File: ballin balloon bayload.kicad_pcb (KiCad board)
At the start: 4 copper layers, 73 x 86 mm, 13 parts, among them J1 Molex 0510211000, J2 Molex 0532611071, J3 Molex 0510211000, J4 Conn_01x06_Pin, J5 Conn_01x06_Pin, U1 MICROSD_SPI_OR_SDIO_CARD, U2 3073, U3 2472

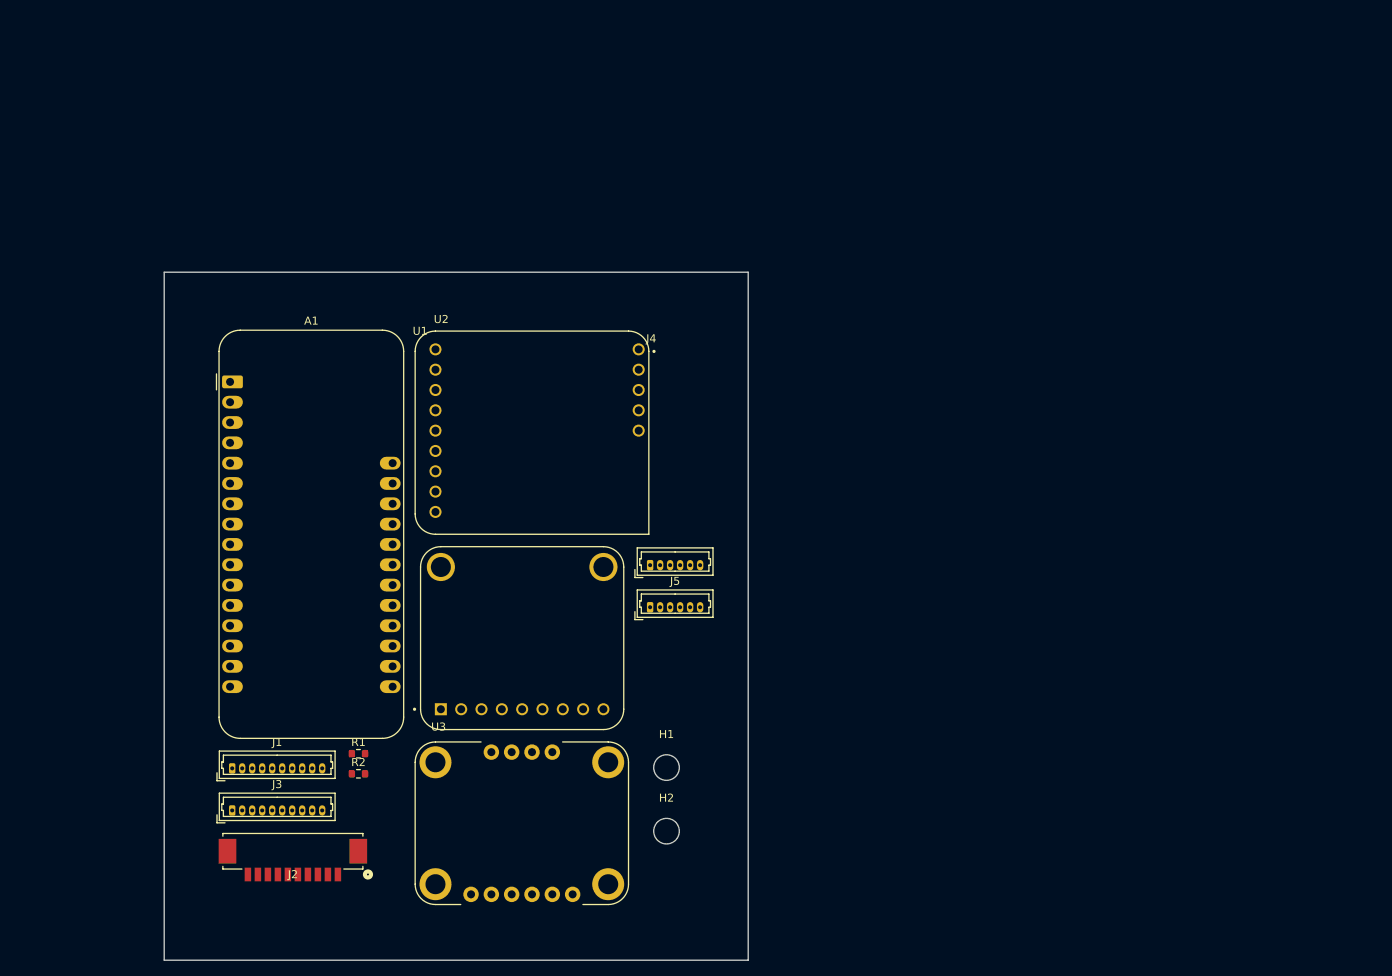
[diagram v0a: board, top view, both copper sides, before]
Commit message: updated pcb layout
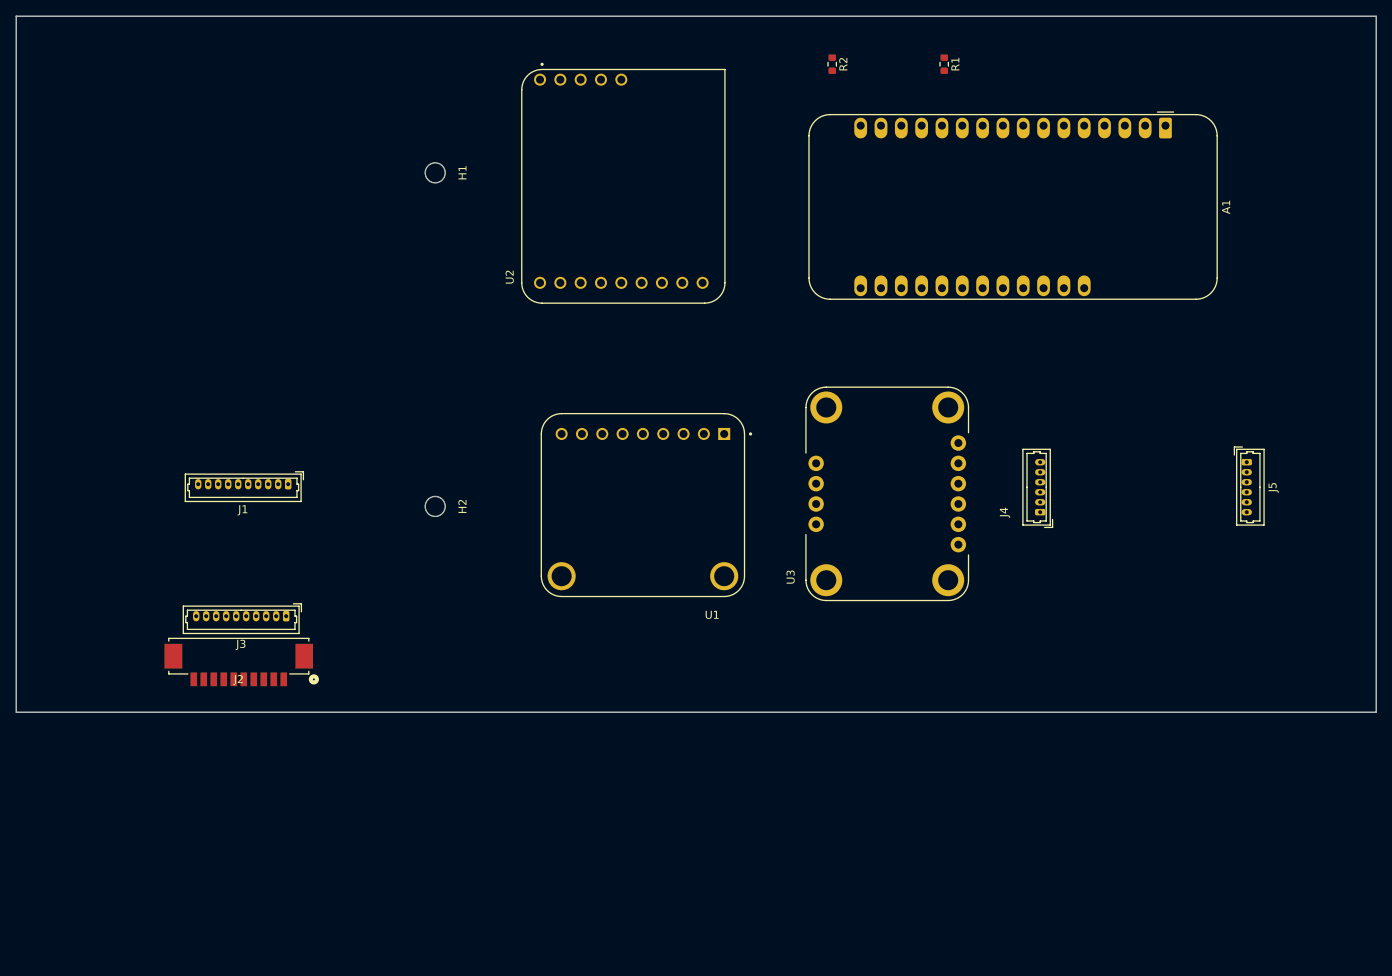
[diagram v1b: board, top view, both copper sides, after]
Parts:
- H1, H2: footprint MountingHole:MountingHole_3.2mm_M3 -> MountingHole:MountingHole_2.5mm
- moved A1 121.2 mm to (190.2, 71.2), turned to -90 degrees
- moved R1 113.1 mm to (162.5, 63.5), turned to -90 degrees
- moved R2 106.7 mm to (148.5, 63.5), turned to -90 degrees
- moved H1 79.8 mm to (98.9, 77.1), turned to -90 degrees
- moved J5 76.8 mm to (200.3, 113.2), turned to -90 degrees
- moved U3 61.5 mm to (155.4, 117.2), turned to 90 degrees
- moved H2 49.8 mm to (98.9, 118.8), turned to -90 degrees
- moved J4 49.2 mm to (174.5, 119.5), turned to 90 degrees
- moved J1 36.2 mm to (80.5, 116.0), turned to 180 degrees
- moved U2 32.8 mm to (122.4, 78.8), turned to 90 degrees
- moved J2 25.3 mm to (74.3, 137.5)
- moved J3 25.2 mm to (80.2, 132.5), turned to 180 degrees
- moved U1 22.5 mm to (124.8, 118.6), turned to 180 degrees
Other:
- board size 73 x 86 mm -> 170 x 87 mm
